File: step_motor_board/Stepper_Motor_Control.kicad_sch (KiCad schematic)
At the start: 57 parts, among them J2 DG141R-2.54-10P-14-00A(H) (Dr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, Q1 2SC2712 (SOT-23), Q2 2SC2712 (SOT-23), Q3 2SC2712 (SOT-23), U4 Pai141M30 (SOIC-16), U6 L78L05 (SOT89-3), U8 74LVC2G14 (SOT-23-6)

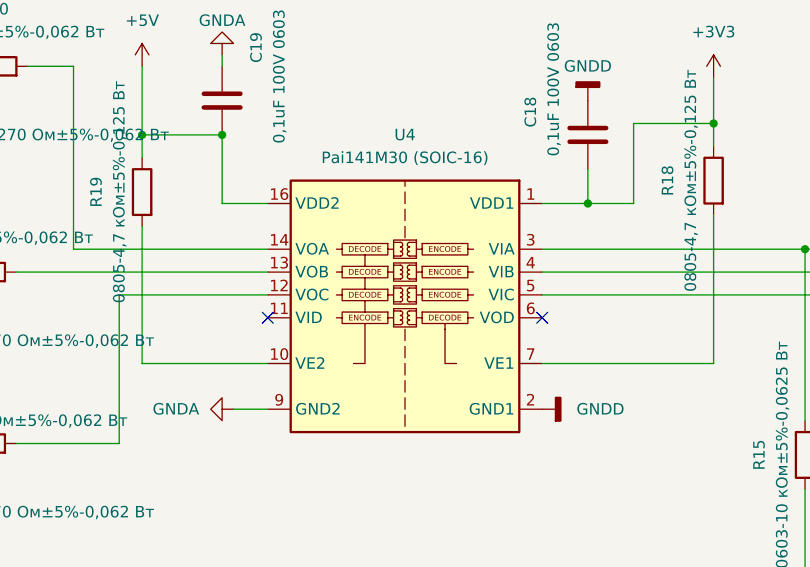
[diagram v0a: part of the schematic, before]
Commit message: update schemas
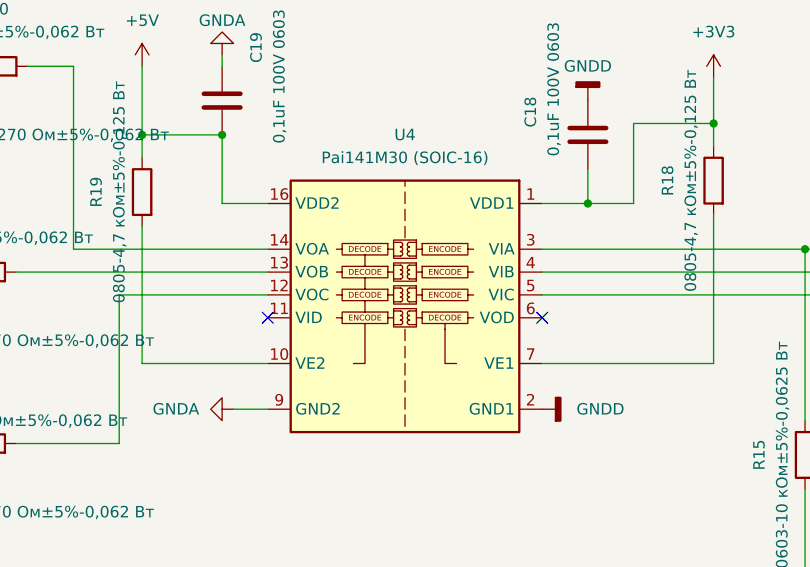
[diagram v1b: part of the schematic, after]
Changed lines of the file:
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@@
 (kicad_sch
-	(version 20231120)
+	(version 20250114)
 	(generator "eeschema")
-	(generator_version "8.0")
+	(generator_version "9.0")
 	(paper "A4")
 	(junction
@@
 	(label "EN_out-"
 		(at 30.48 41.91 0)
-		(fields_autoplaced yes)
 		(effects
 			(font
@@
 	(label "IN_POSITION"
 		(at 232.41 133.35 0)
-		(fields_autoplaced yes)
 		(effects
 			(font
@@
 	(label "IN_POSITION_out+"
 		(at 85.09 54.61 0)
-		(fields_autoplaced yes)
 		(effects
 			(font
@@
 	(label "DIR"
 		(at 254 50.8 0)
-		(fields_autoplaced yes)
 		(effects
 			(font
@@
 	(label "ALARM_out+"
 		(at 57.15 124.46 180)
-		(fields_autoplaced yes)
 		(effects
 			(font
@@
 	(label "ALARM_out+"
 		(at 88.9 59.69 0)
-		(fields_autoplaced yes)
 		(effects
 			(font
@@
 	(label "EN_out-"
 		(at 113.03 22.86 180)
-		(fields_autoplaced yes)
 		(effects
 			(font
@@
 	(label "DIR_out-"
 		(at 111.76 45.72 180)
-		(fields_autoplaced yes)
 		(effects
 			(font
@@
 	(label "STEP_out-"
 		(at 113.03 64.77 180)
-		(fields_autoplaced yes)
 		(effects
 			(font
@@
 	(label "EN"
 		(at 254 48.26 0)
-		(fields_autoplaced yes)
 		(effects
 			(font
@@
 	(label "IN_POSITION_out+"
 		(at 57.15 135.89 180)
-		(fields_autoplaced yes)
 		(effects
 			(font
@@
 	(label "DIR_out-"
 		(at 30.48 46.99 0)
-		(fields_autoplaced yes)
 		(effects
 			(font
@@
 	(label "STEP_out-"
 		(at 30.48 52.07 0)
-		(fields_autoplaced yes)
 		(effects
 			(font
@@
 	(label "STEP"
 		(at 254 53.34 0)
-		(fields_autoplaced yes)
 		(effects
 			(font
@@
 	(label "ALARM"
 		(at 232.41 110.49 0)
-		(fields_autoplaced yes)
 		(effects
 			(font
@@
 		(shape input)
 		(at 264.16 48.26 0)
-		(fields_autoplaced yes)
 		(effects
 			(font
@@
 		(shape input)
 		(at 255.27 133.35 0)
-		(fields_autoplaced yes)
 		(effects
 			(font
@@
 		(shape input)
 		(at 264.16 50.8 0)
-		(fields_autoplaced yes)
 		(effects
 			(font
@@
 		(shape input)
 		(at 264.16 53.34 0)
-		(fields_autoplaced yes)
 		(effects
 			(font
@@
 		(shape input)
 		(at 255.27 110.49 0)
-		(fields_autoplaced yes)
-		(effects
-			(font
+		(effects
+			(font
